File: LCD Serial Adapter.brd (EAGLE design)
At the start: 45.4 x 21.8 mm, 10 parts, among them IC1 74HC595N, IC2 74LHC95N, IC3 DS1866, IC4 MAX4544, Q1 BC327

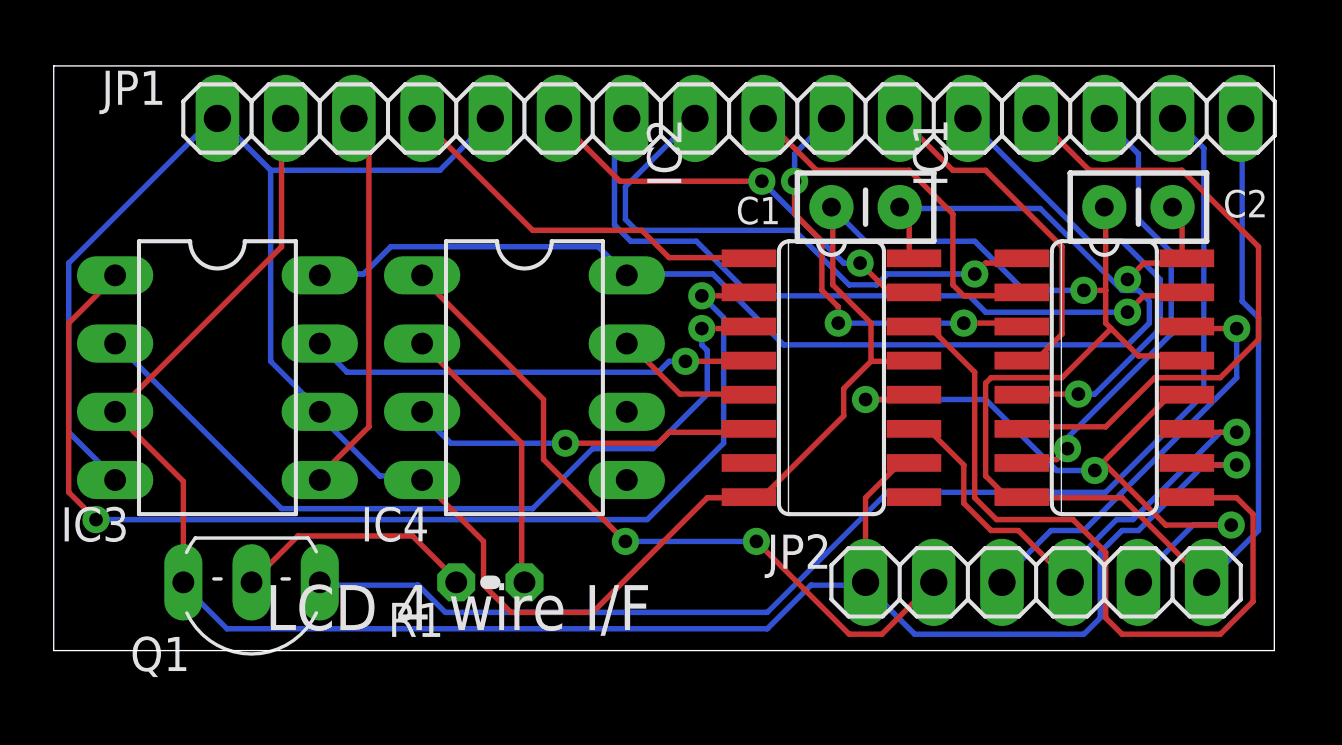
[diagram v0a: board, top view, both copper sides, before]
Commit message: Add files via upload
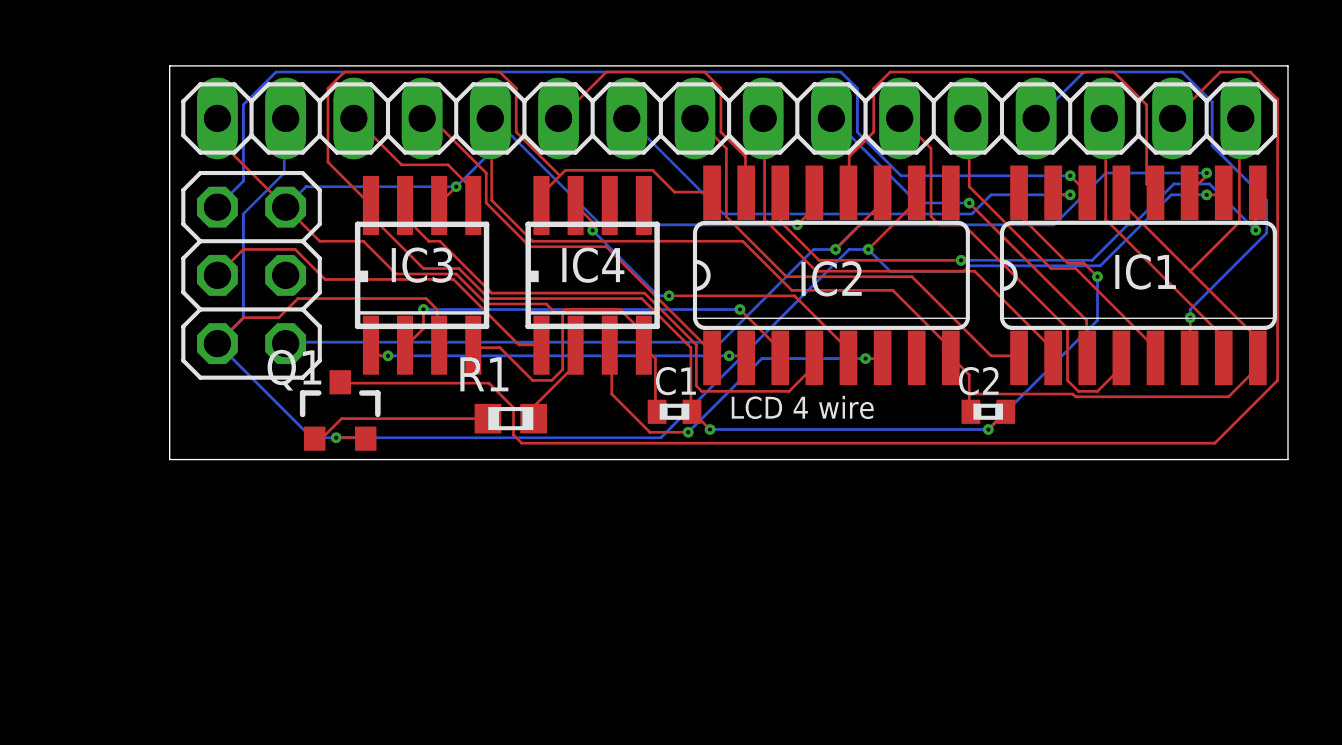
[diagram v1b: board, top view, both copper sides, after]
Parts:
- C1, C2: device SparkFun-Capacitors:CAP-PTH-SMALL2 -> 00 Nik misc:C0402
- IC3: value DS1866 -> DS1866Z; device nik analog ic:DIL-08 -> 00 Nik misc:SOIC8
- IC4: device nik analog ic:DIL-08 -> 00 Nik misc:SOIC8
- JP2: value MCU -> (none); device pinhead:1X06 -> pinhead:2X03
- Q1: value BC327 -> BC807; device transistor-pnp:TO92-EBC -> 00 Nik misc:SOT23-3
- R1: device resistor:0204V -> 00 Nik misc:RES-VERT
- moved JP2 31.4 mm to (27.9, 14.0), turned to 90 degrees
- moved C1 11.3 mm to (43.7, 8.89)
- moved C2 10.3 mm to (55.4, 8.89)
- moved IC3 8.52 mm to (34.3, 14.0), turned to 0 degrees
- moved Q1 8.30 mm to (31.2, 8.89), turned to 0 degrees
- moved R1 6.14 mm to (37.6, 8.64)
- moved IC4 4.58 mm to (40.6, 14.0), turned to 0 degrees
- moved IC1 4.02 mm to (61.0, 14.0), turned to 0 degrees
- moved IC2 3.81 mm to (49.5, 14.0), turned to 0 degrees
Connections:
- net +5V: now also JP2.2, Q1.2; no longer JP2.6, Q1.E
- net BL-PWM: now also JP2.4; no longer JP2.5
- net DATA: now also JP2.6; no longer JP2.4
- net GND: now also JP2.5; no longer JP2.1
- net LATCH: no longer JP2.2
- net LED+: now also Q1.3; no longer Q1.C
- net N$21: now also Q1.1; no longer Q1.B
- net SHIFT: now also JP2.1; no longer JP2.3
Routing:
- net BL-S0: track 42.4 -> 14.2 mm
- net GND: track 131.9 -> 106.4 mm, vias 1 -> 2
- net DATA: track 15.7 -> 38.9 mm
- net SHIFT: track 19.9 -> 40.7 mm, vias 1 -> 2
- net BL-S1: track 30.6 -> 15.9 mm, vias 1 -> 2
- net BL-PWM: track 26.7 -> 13.9 mm, vias 2 -> 0
- net VCC: track 52.2 -> 65.0 mm, vias 1 -> 3
- net VO: track 14.5 -> 6.12 mm
- net DB0: track 27.1 -> 19.0 mm
- net LATCH: track 26.3 -> 18.6 mm, vias 3 -> 0
- net BL-SEL: track 5.31 -> 12.9 mm, vias 0 -> 2
- net BL-DRV: track 10.5 -> 3.41 mm
- net +5V: track 73.9 -> 67.3 mm, vias 1 -> 3
- net DB7: track 16.9 -> 10.8 mm, vias 1 -> 0
- net N$7: track 28.0 -> 22.7 mm, vias 0 -> 2
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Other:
- board size 45.4 x 21.8 mm -> 41.6 x 14.7 mm
- board text added: "LCD 4 wire"

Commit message: Fix contrast signal names
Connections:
- net BL-S0 renamed CON-S0
- net BL-S1 renamed CON-S1
- net BL-S2 renamed CON-S2
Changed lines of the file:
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@@
 <wire x1="45.0088" y1="10.9728" x2="45.085" y2="10.8966" width="0.1016" layer="1"/>
 </signal>
-<signal name="BL-S0">
+<signal name="CON-S0">
 <contactref element="IC2" pad="2"/>
 <contactref element="IC3" pad="1"/>
@@
 <via x="33.02" y="10.9728" extent="1-16" drill="0.1524"/>
 </signal>
-<signal name="BL-S1">
+<signal name="CON-S1">
 <contactref element="IC2" pad="3"/>
 <contactref element="IC3" pad="2"/>
@@
 <wire x1="62.2808" y1="19.812" x2="62.23" y2="19.812" width="0.1016" layer="1"/>
 </signal>
-<signal name="BL-S2">
+<signal name="CON-S2">
 <contactref element="IC3" pad="7"/>
 <contactref element="IC2" pad="4"/>
